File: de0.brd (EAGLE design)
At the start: 150.7 x 90.7 mm, 137 parts, among them IC1 PL2303SA__LF, J1 JUMPER_IN_50, J2 UX60SC-MB-5ST, J3 REG_OUT_33, U1 P0082, U2 RFM95W-915S2, U3 TPS76201DBVR, U4 TPS76201DBVR, U5 TPS76201DBVR

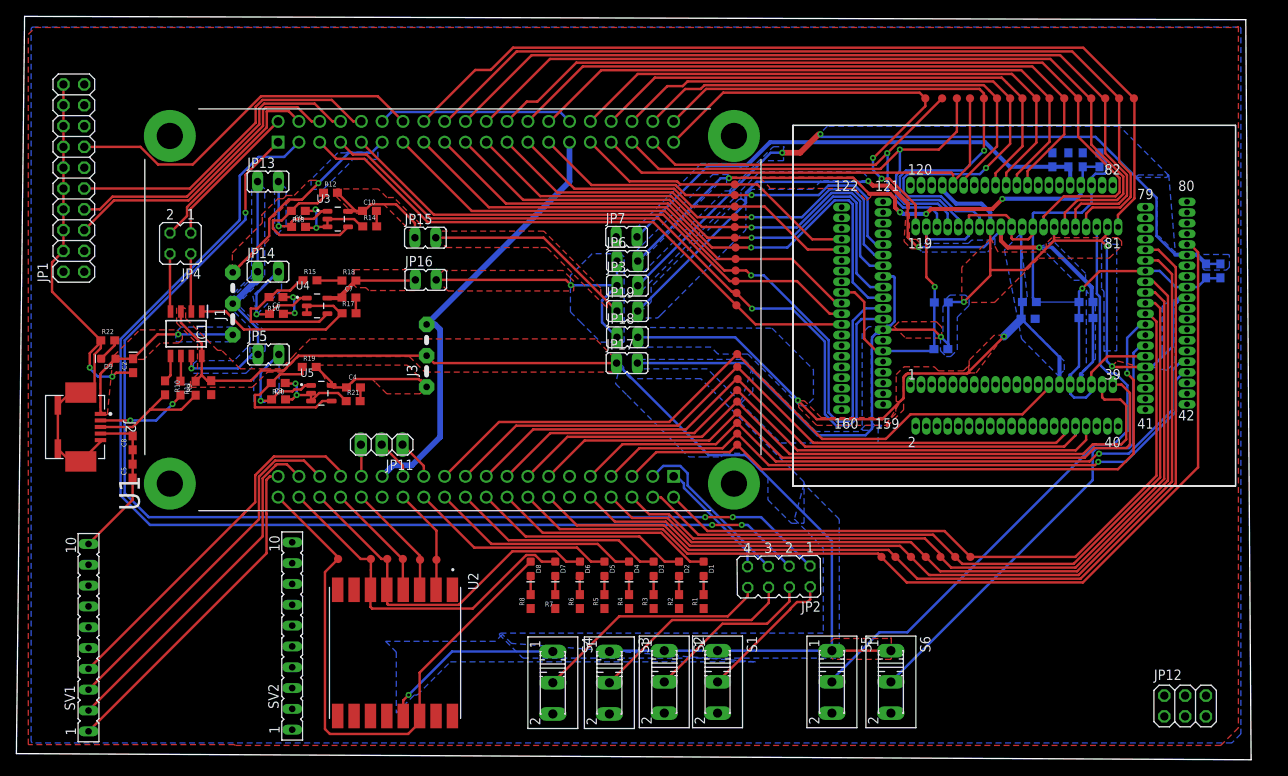
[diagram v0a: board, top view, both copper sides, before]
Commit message: Update layout again
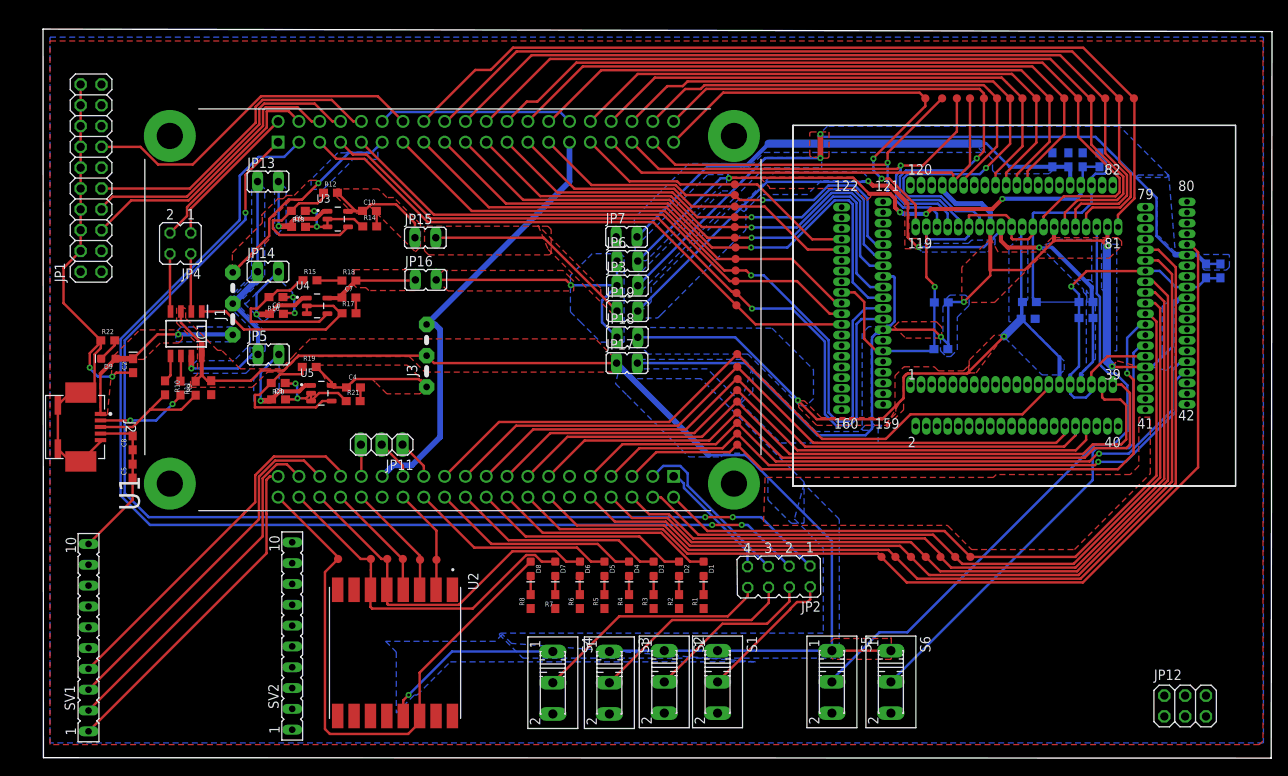
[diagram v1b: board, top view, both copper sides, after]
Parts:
- moved JP1 2.10 mm to (-59.5, 35.9)
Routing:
- net JTAG_TDO: track 44.5 -> 42.4 mm
- net JTAG_TDI: track 36.8 -> 34.7 mm
- net JTAG_TCK: track 40.5 -> 38.4 mm
- net JTAG_TMS: track 38.6 -> 36.7 mm
- net ADDRESS_11: track 61.5 -> 59.6 mm
- net VDD: track 88.4 -> 90.1 mm
- net GND: track 295.4 -> 296.3 mm
- net VDDLS: track 86.6 -> 85.8 mm
- added copper zone on layer 1, net VDD
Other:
- board size 150.7 x 90.7 mm -> 149.9 x 88.9 mm
